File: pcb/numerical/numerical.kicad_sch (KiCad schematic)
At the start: 73 parts, among them J1 AudioJack3_Ground, U1 Raspberry_Pi_Pico

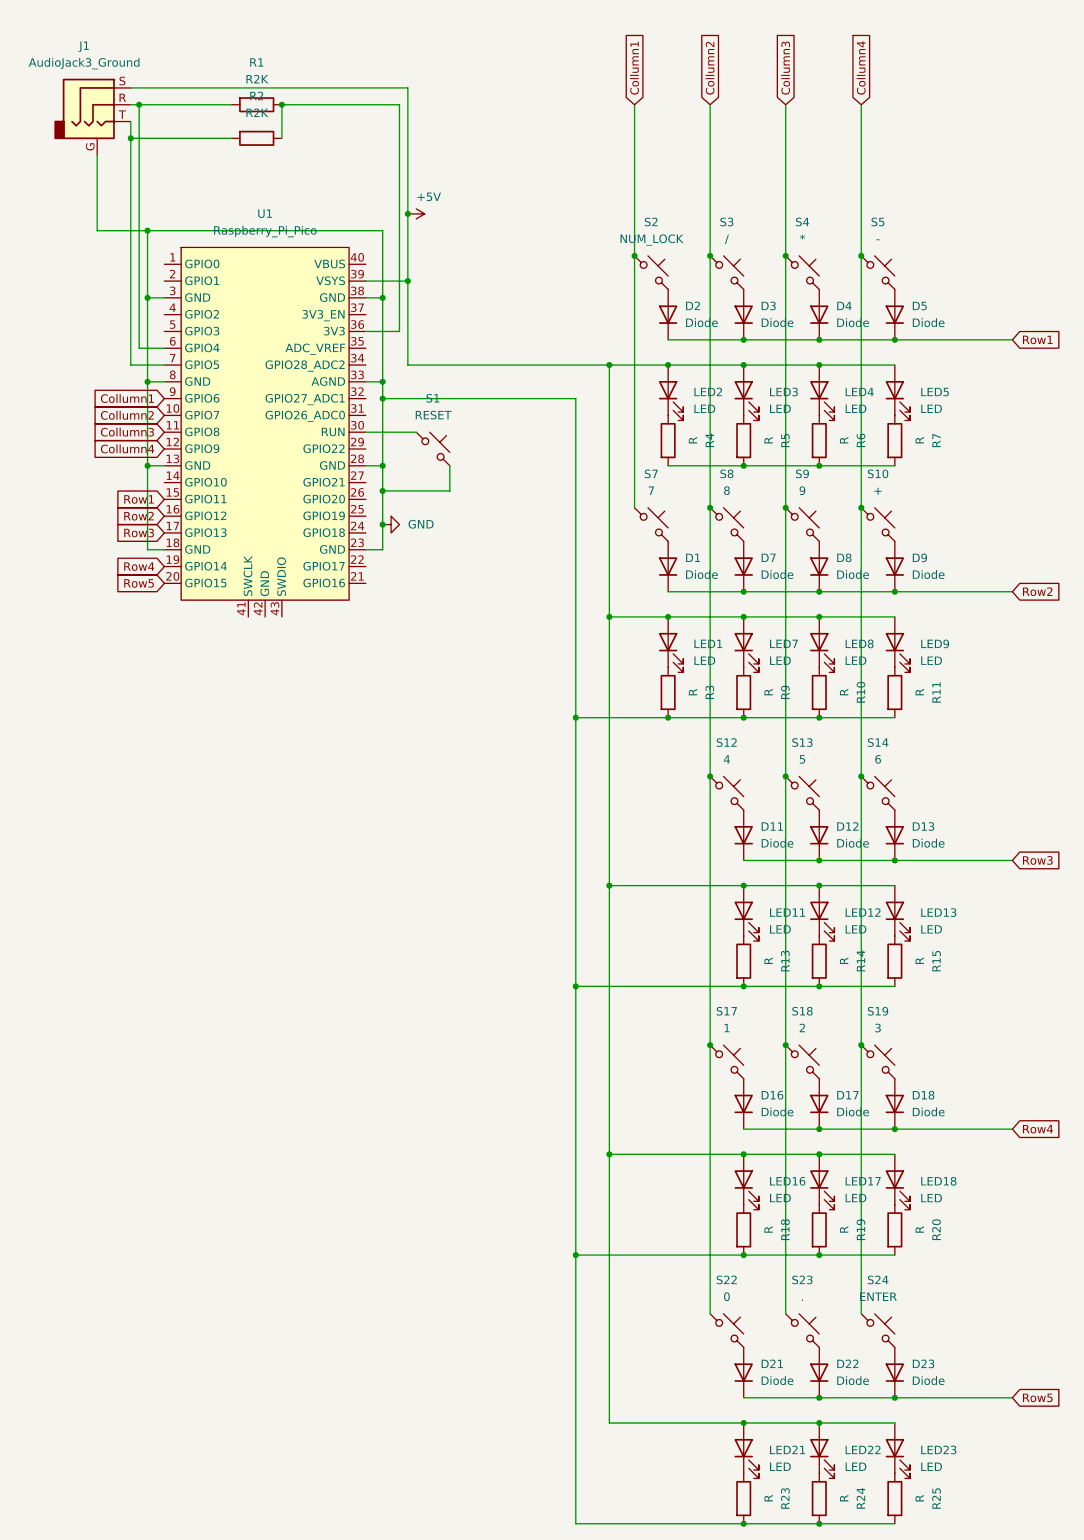
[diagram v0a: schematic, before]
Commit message: numerical done
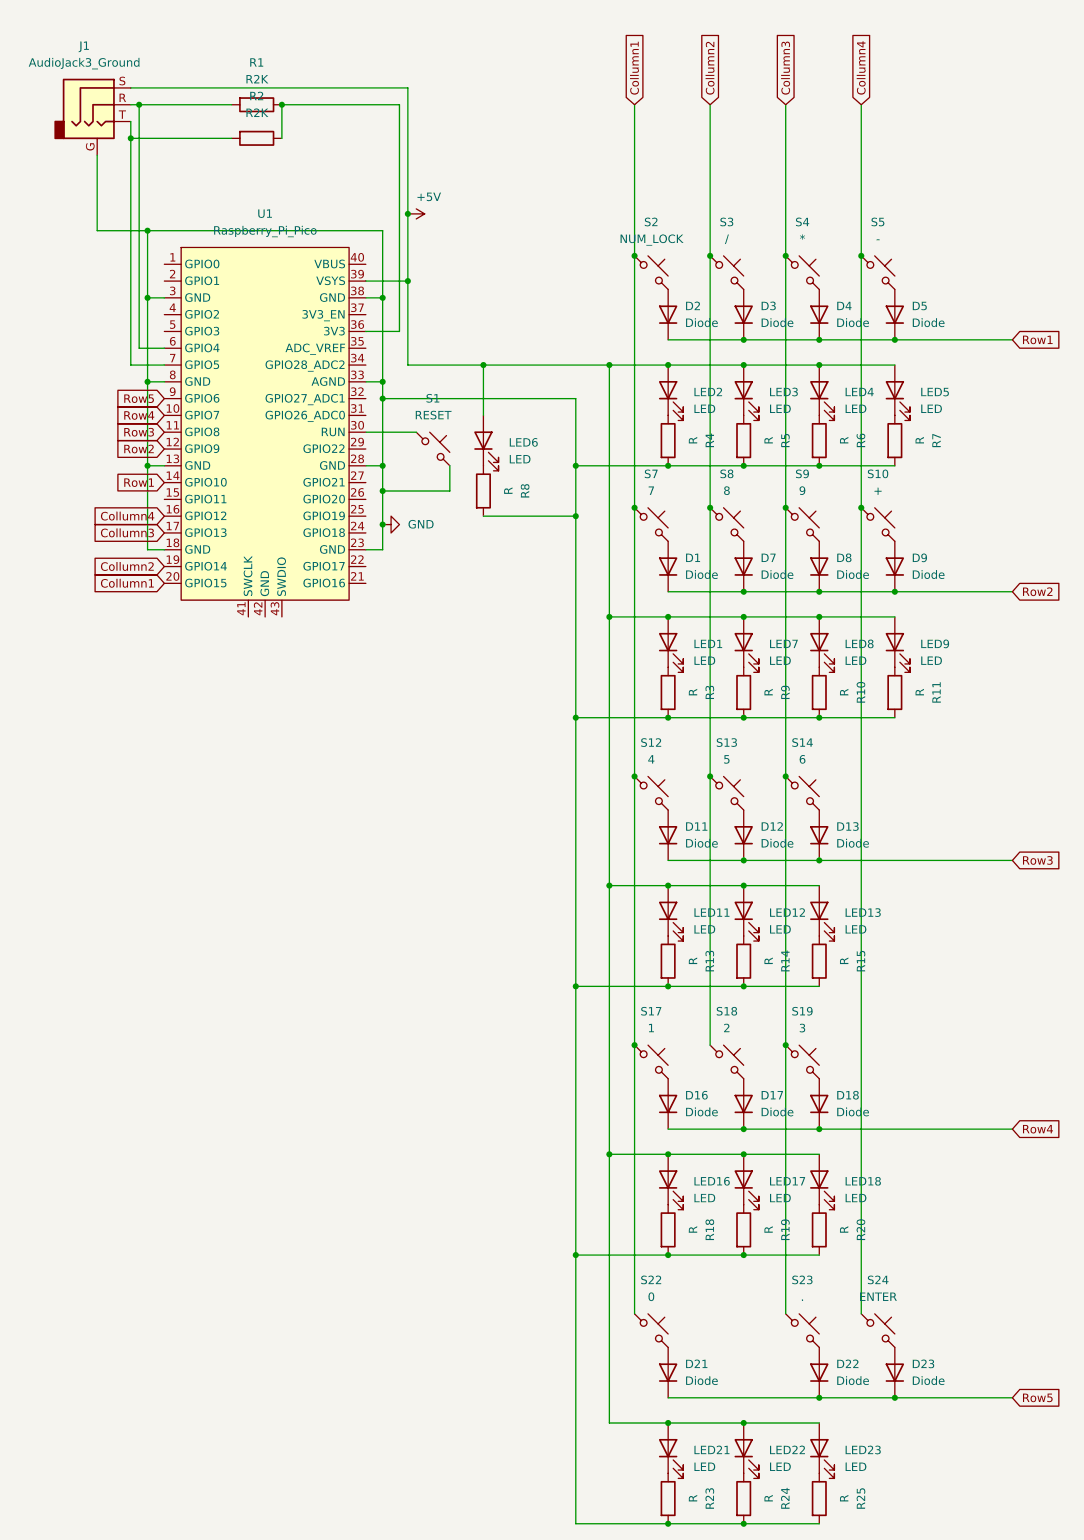
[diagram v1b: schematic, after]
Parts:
- added LED6: LED, MX V2 Misc:MX-LED-PolarityMarked, symbol Device:LED
- added R8: R, Resistor_SMD:R_0603_1608Metric_Pad0.98x0.95mm_HandSolder, symbol Device:R
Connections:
- net +5V: now also LED6.2 (A)
- net Collumn1: now also S12.1, S17.1, S22.1, U1.20 (GPIO15); no longer U1.9 (GPIO6)
- net Collumn2: now also S13.1, S18.1, U1.19 (GPIO14); no longer S12.1, S17.1, S22.1, U1.10 (GPIO7)
- net Collumn3: now also S14.1, S19.1, U1.17 (GPIO13); no longer S13.1, S18.1, U1.11 (GPIO8)
- net Collumn4: now also U1.16 (GPIO12); no longer S14.1, S19.1, U1.12 (GPIO9)
- net GND: now also R4.2, R5.2, R6.2, R7.2, R8.2
- net Row1: now also U1.14 (GPIO10); no longer U1.15 (GPIO11)
- net Row2: now also U1.12 (GPIO9); no longer U1.16 (GPIO12)
- net Row3: now also U1.11 (GPIO8); no longer U1.17 (GPIO13)
- net Row4: now also U1.10 (GPIO7); no longer U1.19 (GPIO14)
- net Row5: now also U1.9 (GPIO6); no longer U1.20 (GPIO15)
- new net: LED6.1 (K), R8.1
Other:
- moved on the sheet: D11, D12, D13, D16, D17, D18, D21, LED11, LED12, LED13, LED16, LED17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
